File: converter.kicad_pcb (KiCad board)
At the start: 2 copper layers, 26 x 37 mm, 61 parts, among them CN1 MINI_DIN_8P_JACK, J1 USB_mini_micro_B, P1 CONN_1, P2 CONN_1, P3 CONN_1, P4 CONN_1, SW1 SW_PUSH, U1 32U2, X1 16MHz

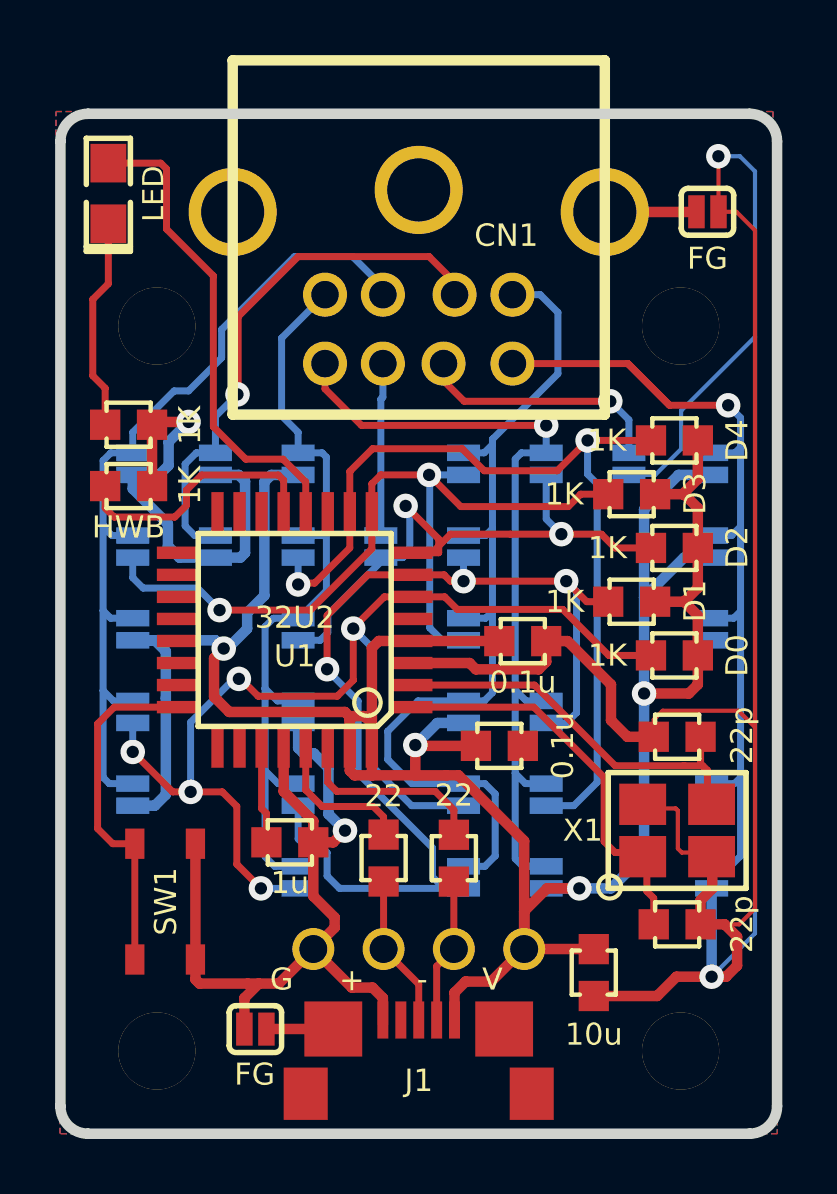
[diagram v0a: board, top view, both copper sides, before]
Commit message: rev2.1
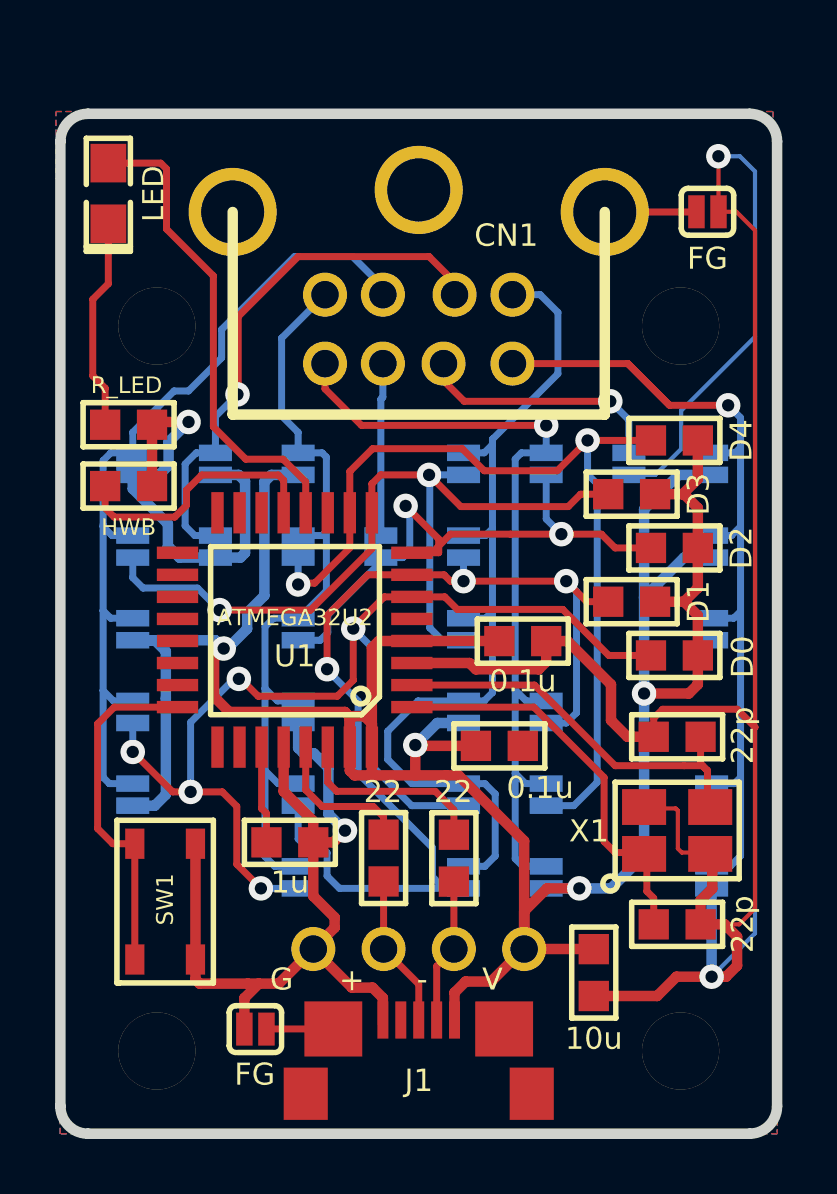
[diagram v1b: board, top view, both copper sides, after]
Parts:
- R3: value 1K -> 1k
- R4: value 1K -> R_LED
- U1: value 32U2 -> ATMEGA32U2
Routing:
- net Net-(J1-Pad6): track 4.86 -> 2.43 mm
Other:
- rule pad_to_mask_clearance: 0.254 -> 0.1
